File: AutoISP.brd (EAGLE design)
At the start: 26.6 x 15.2 mm, 7 parts

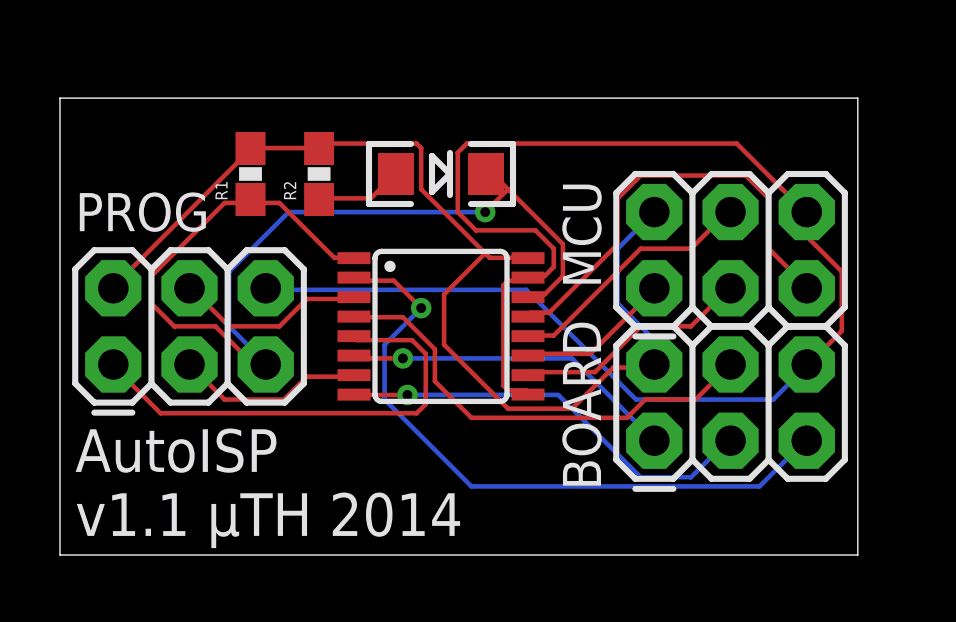
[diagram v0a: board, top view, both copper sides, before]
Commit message: Revise boards for better labelling and sane orientation, add AutoISP328
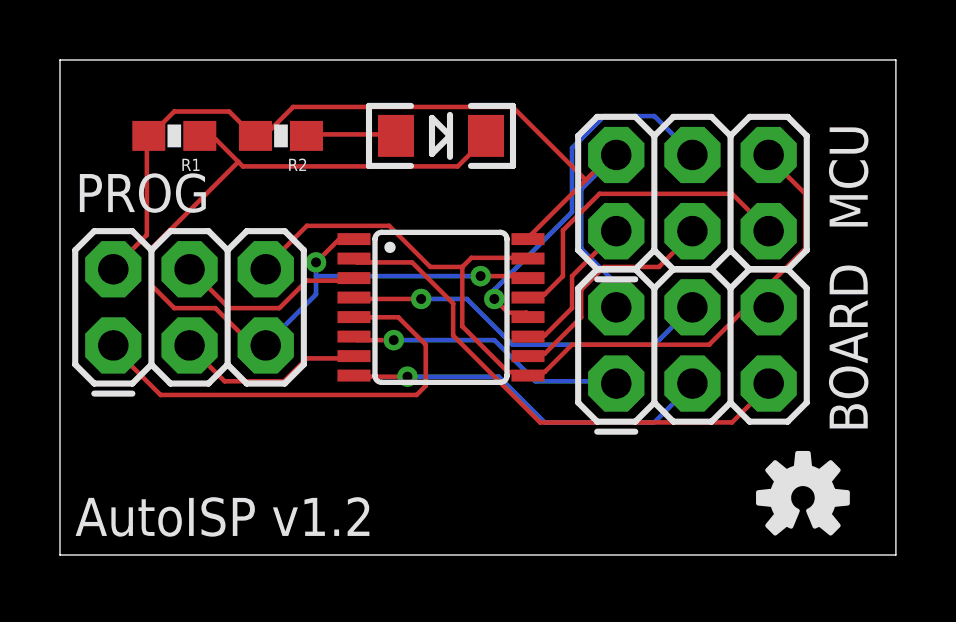
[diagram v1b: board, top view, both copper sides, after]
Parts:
- added LOGO1: OSHW-LOGOS, SparkFun-Aesthetics:OSHW-LOGO-S
- moved R1 2.84 mm to (3.81, 14.0), turned to 180 degrees
- moved BOARD 2.29 mm to (18.5, 5.71)
- moved MCU 2.29 mm to (18.5, 10.8)
- moved R2 1.80 mm to (7.37, 14.0), turned to 180 degrees
- moved LED1 1.27 mm to (12.7, 14.0)
- moved PROG 0.64 mm to (1.78, 6.99)
- moved U$1 0.64 mm to (12.7, 8.26)
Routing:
- net N$6: track 51.5 -> 30.0 mm
- net N$5: track 22.1 -> 17.3 mm, vias 1 -> 0
- net N$7: track 36.5 -> 31.8 mm
- net N$12: track 8.46 -> 12.5 mm, vias 0 -> 1
- net N$11: track 14.7 -> 10.9 mm
- net N$8: track 15.3 -> 12.4 mm, vias 0 -> 1
- net N$1: track 34.4 -> 32.5 mm, vias 1 -> 2
- net N$9: track 11.2 -> 9.39 mm
- net N$10: track 14.2 -> 12.5 mm
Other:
- board size 26.6 x 15.2 mm -> 27.9 x 16.5 mm
- board text added: "*"
- board text added: "AutoISP v1.2"
- board text added: "µTH '15 CC BY"
- board text removed: "AutoISP v1.1 µTH 2014"
